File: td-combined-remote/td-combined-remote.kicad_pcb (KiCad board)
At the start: 2 copper layers, 80 x 30 mm, 18 parts, among them J1 Conn_01x10_Pin, J2 Conn_01x06_Pin

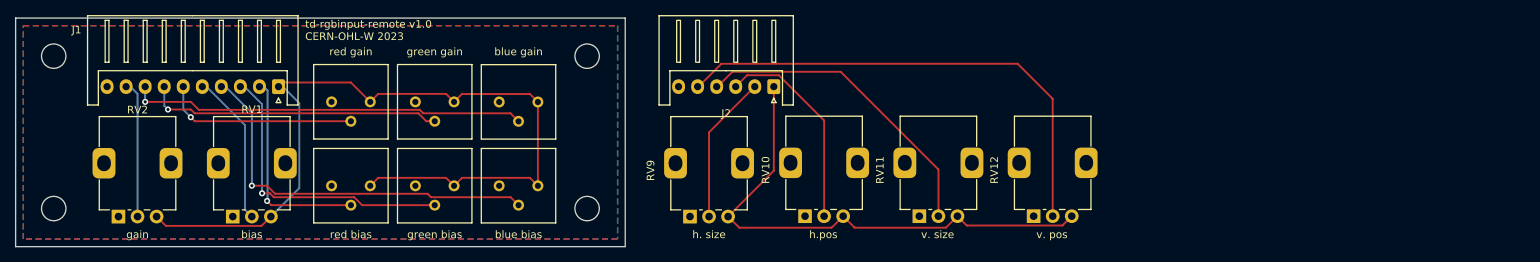
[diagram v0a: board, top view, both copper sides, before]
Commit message: bunch of random updates
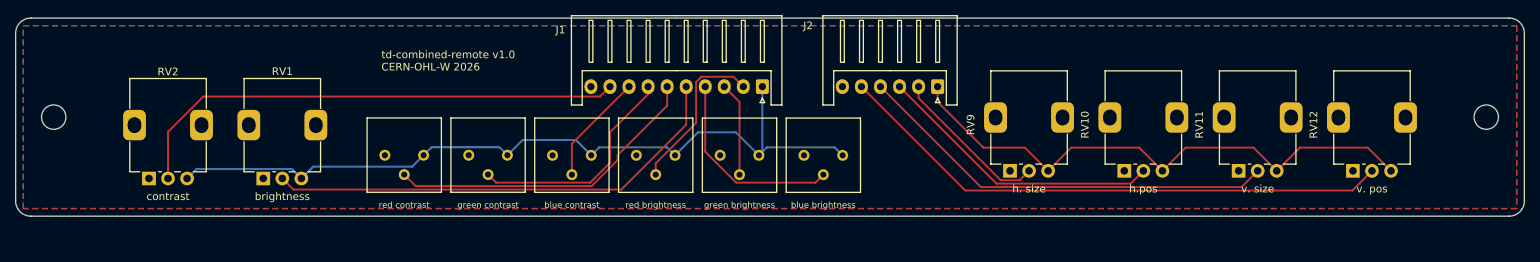
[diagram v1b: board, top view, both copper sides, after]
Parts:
- removed H2, H4: MountingHole, MountingHole:MountingHole_3.2mm_M3
- moved H3 188.4 mm to (311.0, 75.0)
- moved J1 63.5 mm to (216.0, 71.0)
- moved RV9 42.4 mm to (248.5, 82.0)
- moved RV10 42.3 mm to (263.5, 82.0)
- moved RV11 42.3 mm to (278.5, 82.0)
- moved RV12 42.3 mm to (293.5, 82.0)
- moved RV3 40.2 mm to (199.5, 80.0)
- moved RV4 40.2 mm to (210.5, 80.0)
- moved RV5 40.2 mm to (221.5, 80.0)
- moved J2 21.5 mm to (239.0, 71.0)
- moved RV6 9.90 mm to (166.5, 80.0)
- moved RV7 9.90 mm to (177.5, 80.0)
- moved RV8 9.90 mm to (188.5, 80.0)
- moved H1 8.00 mm to (123.0, 75.0)
- moved RV1 6.40 mm to (150.5, 83.0)
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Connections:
- J2 pad 1: +3.3VA -> +3.3V
- RV10 pad 3: +3.3VA -> +3.3V
- RV11 pad 3: +3.3VA -> +3.3V
- RV12 pad 3: +3.3VA -> +3.3V
- RV9 pad 3: +3.3VA -> +3.3V
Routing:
- net +3.3V: track 0.00 -> 72.8 mm
- net +3.3VA: track 176.0 -> 104.3 mm
- net /globalgain: track 18.2 -> 66.6 mm
- net /globalbias: track 20.3 -> 62.1 mm
- net /bgain: track 52.6 -> 14.7 mm, vias 1 -> 0
- net /gbias: track 39.0 -> 12.4 mm, vias 1 -> 0
- net /bbias: track 51.3 -> 26.2 mm, vias 1 -> 0
- net /rgain: track 26.2 -> 42.4 mm, vias 1 -> 0
- net /vsize: track 41.3 -> 55.8 mm
- net /hpos: track 27.2 -> 38.0 mm
- net /ggain: track 39.4 -> 29.6 mm, vias 1 -> 0
- net /vpos: track 65.1 -> 73.7 mm
- net /rbias: track 27.2 -> 21.4 mm, vias 1 -> 0
- net /hsize: track 19.5 -> 21.0 mm
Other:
- board size 80 x 30 mm -> 198 x 26 mm
- board text added: "blue brightness"
- board text added: "blue contrast"
- board text added: "brightness"
- board text added: "contrast"
- board text added: "green brightness"
- board text added: "green contrast"
- board text added: "red brightness"
- board text added: "red contrast"
- board text added: "td-combined-remote v1.0 CERN-OHL-W 2026"
- board text removed: "bias"
- board text removed: "blue bias"
- board text removed: "blue gain"
- board text removed: "gain"
- board text removed: "green bias"
- board text removed: "green gain"
- board text removed: "red bias"
- board text removed: "red gain"
- board text removed: "td-rgbinput-remote v1.0 CERN-OHL-W 2023"
